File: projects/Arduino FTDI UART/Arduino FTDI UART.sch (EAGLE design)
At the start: 19 parts, among them IC1 FT232RL, X1 MINI-USB, X2 USB-A-SHIELD

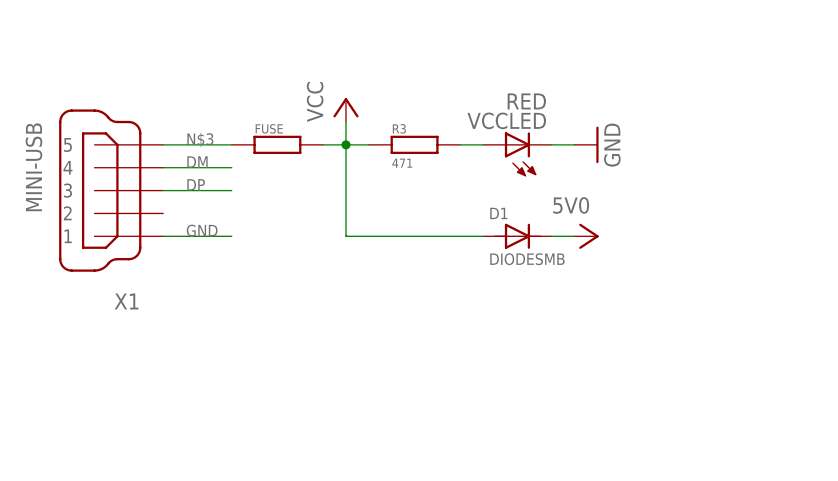
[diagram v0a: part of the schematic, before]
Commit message: 2020.06.01.01
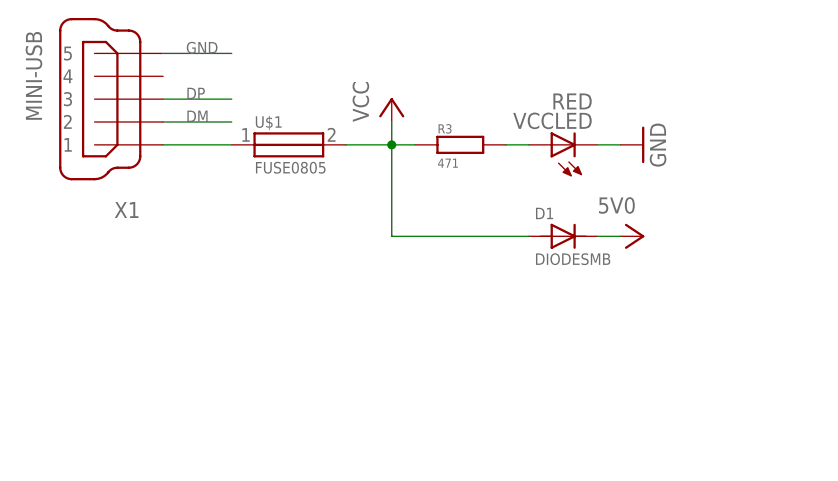
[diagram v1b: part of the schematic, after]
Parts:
- removed FUSE: RR0805, RCLDA:RR0805
- added U$1: FUSE0805, RCLDA:FUSE0805
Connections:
- net DM: now also X1.2; no longer X1.4
- net GND: now also X1.5; no longer X1.1
- net N$3: now also U$1.P$1, X1.1; no longer FUSE.1, X1.5
- net VCC: now also U$1.P$2; no longer FUSE.2
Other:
- moved on the sheet: D1, R3, VCCLED, X1
